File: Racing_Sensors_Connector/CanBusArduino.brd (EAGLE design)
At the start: 48.3 x 43.2 mm, 26 parts, among them U2 SPARKFUN_USD-SOCKETSMD, U3 AT90CAN128-16AI

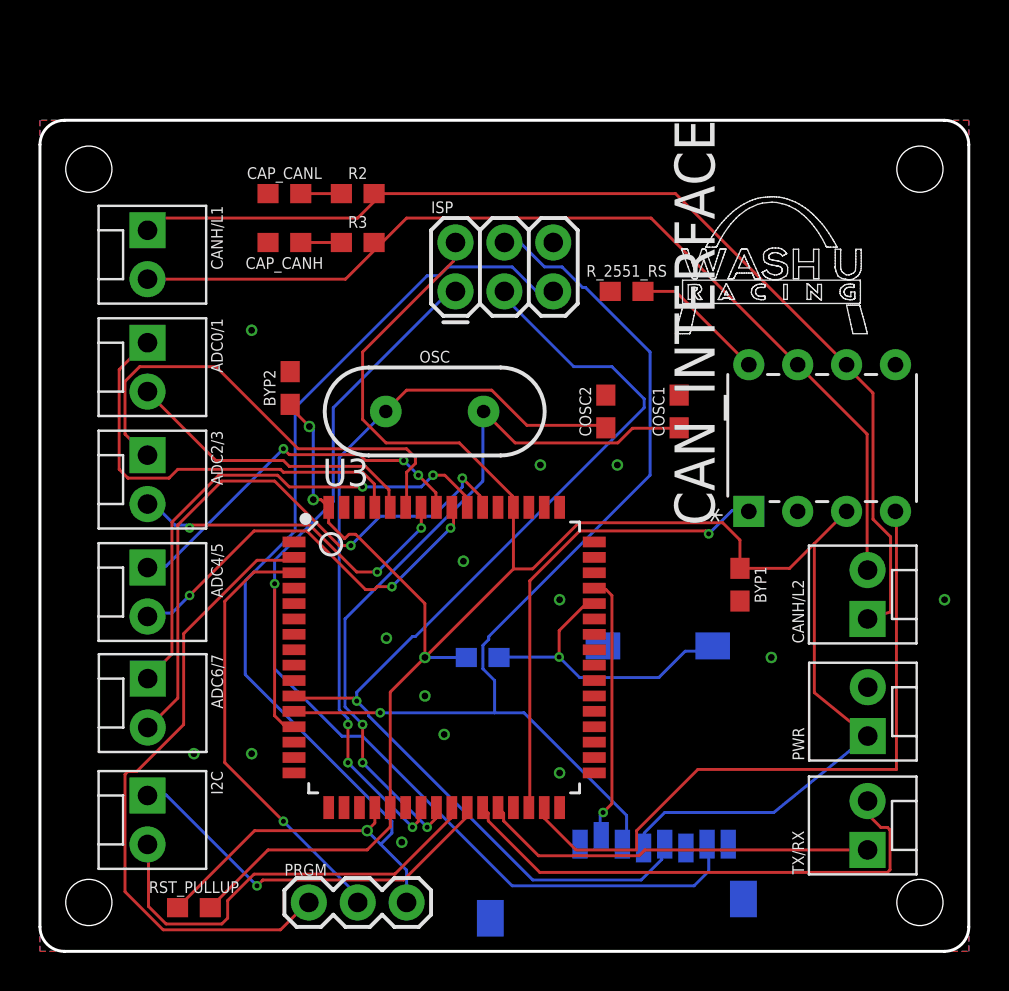
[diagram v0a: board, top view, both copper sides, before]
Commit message: Before SD fix
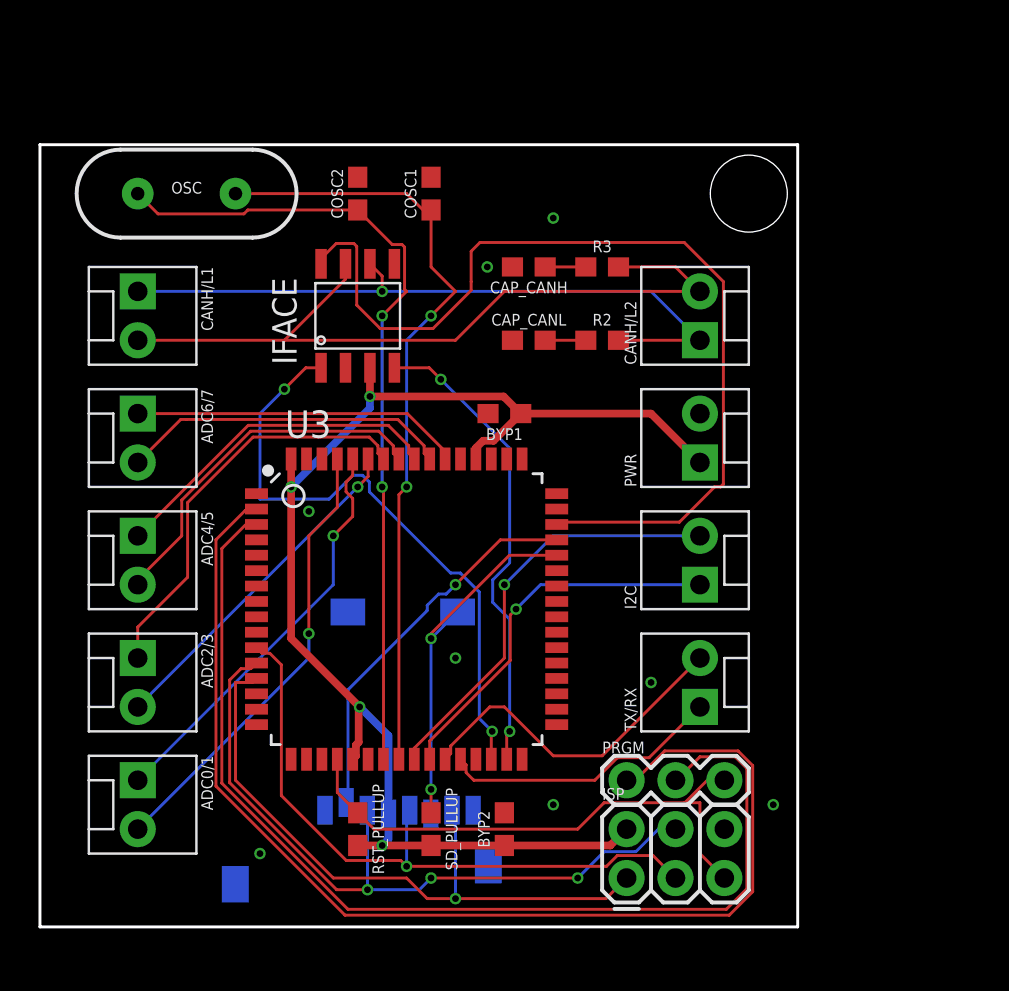
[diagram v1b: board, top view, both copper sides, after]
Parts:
- removed CAN_INTERFACE: MCP2551-I/P, can_transceiver:DIP254P762X432-8
- removed R_2551_RS: 4.7k, SparkFun-Resistors:0603
- added IFACE: MCP2561-E/SN, Volks73-MicrochipTechnology:SOIC-8
- moved ISP 31.8 mm to (30.5, 2.54)
- moved I2C 30.7 mm to (34.3, 17.8), turned to 90 degrees
- moved BYP2 25.5 mm to (24.1, 5.08)
- moved ADC0/1 22.7 mm to (5.08, 7.62)
- moved PRGM 17.7 mm to (30.5, 7.62)
- moved COSC1 17.2 mm to (20.3, 38.1)
- moved COSC2 17.2 mm to (16.5, 38.1)
- moved OSC 17.2 mm to (7.62, 38.1)
- moved CANH/L2 16.9 mm to (34.3, 30.5)
- moved PWR 16.7 mm to (34.3, 24.1)
- moved BYP1 15.1 mm to (24.1, 26.7), turned to 180 degrees
- moved CAP_CANL 14.8 mm to (25.4, 30.5)
- moved R2 14.8 mm to (29.2, 30.5)
- moved ADC6/7 13.8 mm to (5.08, 26.7)
- moved U2 13.4 mm to (23.7, 16.8)
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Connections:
- removed net CI_RS: CAN_INTERFACE.8, R_2551_RS.2
- new net CAN_STBY: IFACE.8, U3.46
- net A0: now also ADC0/1.2; no longer ADC0/1.1
- net A1: now also ADC0/1.1; no longer ADC0/1.2
- net A2: now also ADC2/3.2; no longer ADC2/3.1
- net A3: now also ADC2/3.1; no longer ADC2/3.2
- net A4: now also ADC4/5.2; no longer ADC4/5.1
- net A5: now also ADC4/5.1; no longer ADC4/5.2
- net A6: now also ADC6/7.2; no longer ADC6/7.1
- net A7: now also ADC6/7.1; no longer ADC6/7.2
- net CANH: now also IFACE.7; no longer CAN_INTERFACE.7
- net CANL: now also IFACE.6; no longer CAN_INTERFACE.6
- net CAN_RXD: now also IFACE.4; no longer CAN_INTERFACE.4
- net CAN_TXD: now also IFACE.1; no longer CAN_INTERFACE.1
- net GND: now also IFACE.2; no longer CAN_INTERFACE.2, R_2551_RS.1
- net VCC: now also IFACE.3; no longer CAN_INTERFACE.3
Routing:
- net CAN_STBY: track 0.00 -> 49.1 mm
- net VCC: track 117.6 -> 69.6 mm, vias 3 -> 4
- net TX: track 22.7 -> 55.7 mm, vias 1 -> 0
- net RESET: track 61.6 -> 28.9 mm, vias 1 -> 0
- net RX: track 33.3 -> 60.8 mm
- net MISO: track 60.8 -> 34.2 mm
- net SCK: track 56.3 -> 34.2 mm
- net CANL: track 56.1 -> 36.2 mm, vias 0 -> 1
- net MOSI: track 53.6 -> 38.0 mm, vias 1 -> 3
- net A7: track 32.0 -> 17.2 mm, vias 2 -> 0
- net CAN_RXD: track 35.3 -> 24.7 mm, vias 0 -> 2
- net CANH: track 50.8 -> 40.3 mm
- net RX1: track 27.4 -> 17.8 mm
- net A6: track 26.5 -> 17.2 mm, vias 2 -> 0
- net CAN_TXD: track 24.8 -> 32.3 mm, vias 1 -> 2
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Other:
- board size 48.3 x 43.2 mm -> 39.4 x 40.6 mm
- board text added: "+"
- board text added: "7 6 5 4 3 2 1 0"
- board text added: "CAN Communicator WashU Racing 2018-19"
- board text added: "Connor Monahan"
- board text added: "H L"
- board text added: "L H"
- board text added: "RX1"
- board text added: "SCL"
- board text added: "SDA"
- board text added: "TX1"
- board text removed: "Design: Connor Monahan"
- board text removed: "Ethan Shry"
- board text removed: "WASHU RACING 2017-18"
